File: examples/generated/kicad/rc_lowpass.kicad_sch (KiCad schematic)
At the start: 3 parts

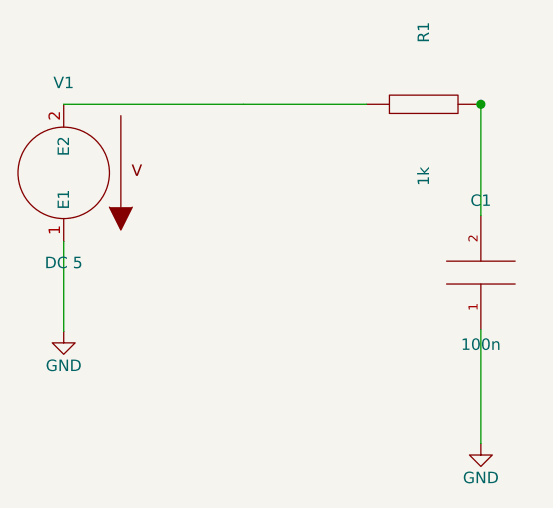
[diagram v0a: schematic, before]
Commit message: Attempt to correct strange wiring.
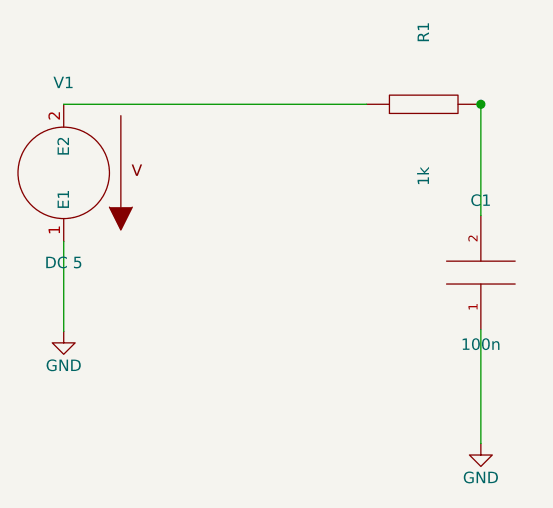
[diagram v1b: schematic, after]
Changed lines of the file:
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@@
     )
   )
-  (wire (pts (xy 50.00 70.38) (xy 70.00 70.38))
+  (wire (pts (xy 50.00 70.38) (xy 83.65 70.38))
     (stroke (width 0) (type solid) (color 0 0 0 0))
   )
-  (wire (pts (xy 83.65 70.38) (xy 70.00 70.38))
-    (stroke (width 0) (type solid) (color 0 0 0 0))
-  )

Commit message: Attempt shape and wiring fixes again.
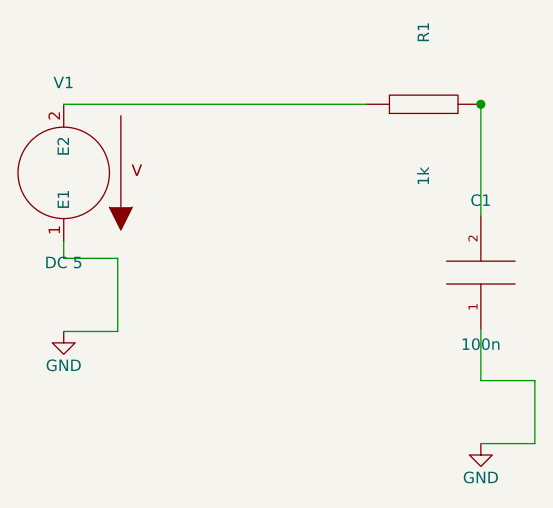
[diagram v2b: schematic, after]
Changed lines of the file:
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@@
     (stroke (width 0) (type solid) (color 0 0 0 0))
   )
-  (wire (pts (xy 50.00 85.62) (xy 50.00 95.62))
+  (wire (pts (xy 50.00 85.62) (xy 50.00 87.50))
     (stroke (width 0) (type solid) (color 0 0 0 0))
   )
-  (wire (pts (xy 96.35 95.43) (xy 96.35 108.08))
+  (wire (pts (xy 50.00 87.50) (xy 56.00 87.50))
     (stroke (width 0) (type solid) (color 0 0 0 0))
   )
+  (wire (pts (xy 56.00 87.50) (xy 56.00 95.62))
+    (stroke (width 0) (type solid) (color 0 0 0 0))
+  )
+  (wire (pts (xy 56.00 95.62) (xy 50.00 95.62))
+    (stroke (width 0) (type solid) (color 0 0 0 0))
+  )
+  (wire (pts (xy 96.35 95.43) (xy 96.35 101.08))
+    (stroke (width 0) (type solid) (color 0 0 0 0))
+  )
+  (wire (pts (xy 96.35 101.08) (xy 102.35 101.08))
+    (stroke (width 0) (type solid) (color 0 0 0 0))
+  )
+  (wire (pts (xy 102.35 101.08) (xy 102.35 108.08))
+    (stroke (width 0) (type solid) (color 0 0 0 0))
+  )
+  (wire (pts (xy 102.35 108.08) (xy 96.35 108.08))
+    (stroke (width 0) (type solid) (color 0 0 0 0))
+  )
